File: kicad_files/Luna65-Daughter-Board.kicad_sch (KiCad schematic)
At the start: 39 parts, among them J1 TYPE-C-31-M12, J2 Molex Power, J3 JSTPH, Q1 TP0610T, U2 USBLC6-2SC6, U3 AP2112, U4 APX803L, U5 TPS61032RSAR, U6 LTC4095

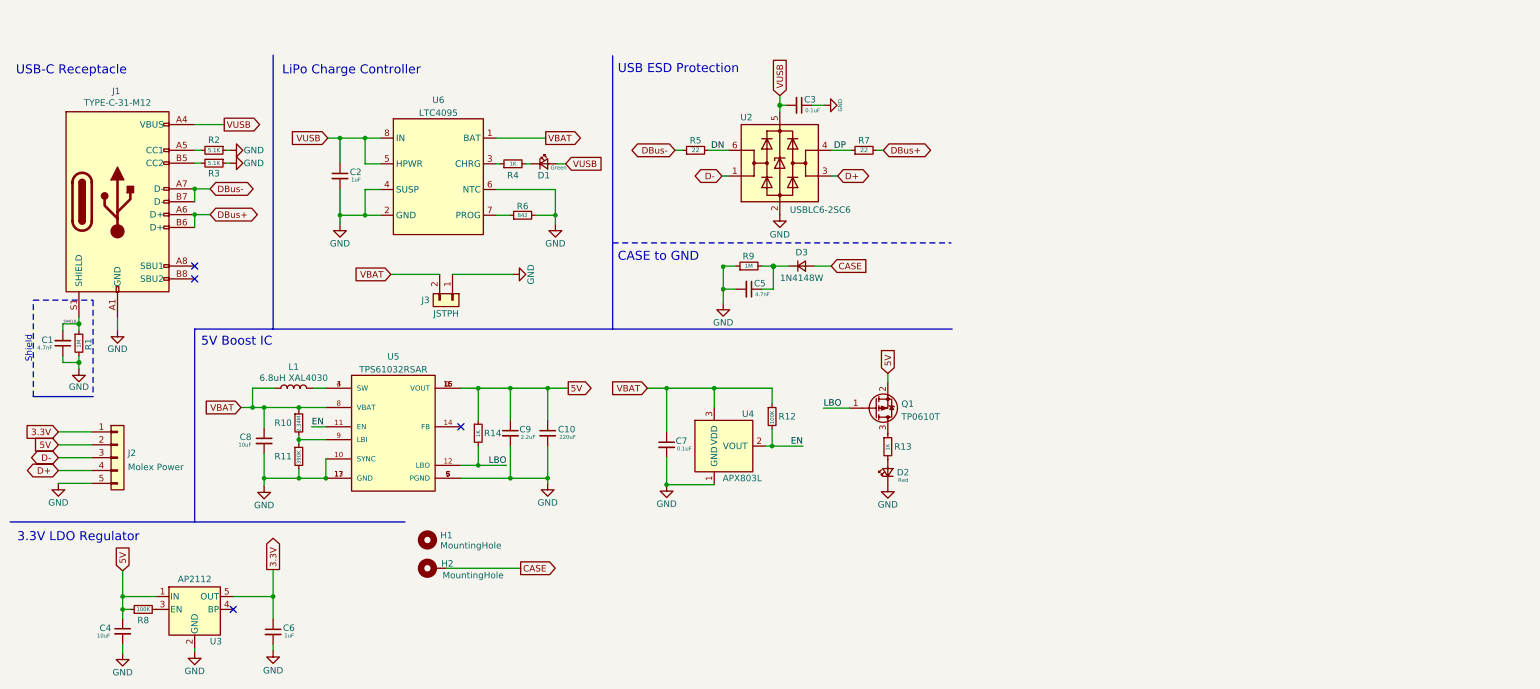
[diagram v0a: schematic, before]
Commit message: stuff
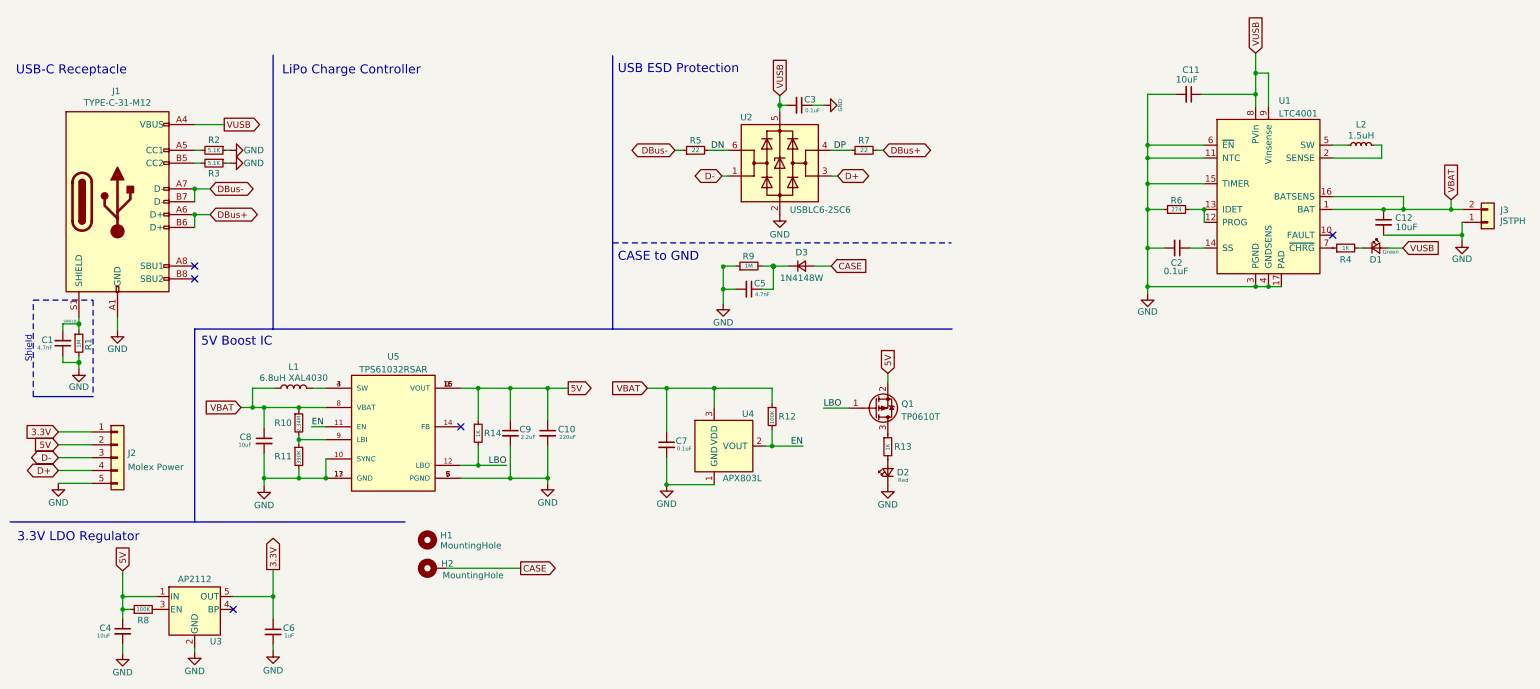
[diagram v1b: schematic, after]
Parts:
- removed U6: LTC4095, Package_DFN_QFN:DFN-8-1EP_2x2mm_P0.5mm_EP0.7x1.3mm, symbol LTC4095:LTC4095
- added C11, C12: 10uF, Capacitor_SMD:C_0603_1608Metric, symbol Device:C_Small
- added L2: 1.5uH, Inductor_SMD:L_0805_2012Metric, symbol Device:L_Small
- added U1: LTC4001, Package_DFN_QFN:QFN-16-1EP_4x4mm_P0.65mm_EP2.15x2.15mm, symbol Battery_Management:LTC4001
- C1, C3, C4, C5, C6, C7, C8, C9: footprint acheron_Components:C_0805_2012Metric -> Capacitor_SMD:C_0603_1608Metric
- C2: value 1uF -> 0.1uF; footprint acheron_Components:C_0805_2012Metric -> Capacitor_SMD:C_0603_1608Metric
- D1, D2: footprint LED_SMD:LED_1206_3216Metric_Pad1.42x1.75mm_HandSolder -> LED_SMD:LED_0805_2012Metric
- R1, R10, R11, R12, R13, R14, R2, R3, R4, R5, R7, R8, R9: footprint Resistor_SMD:R_0805_2012Metric -> Resistor_SMD:R_0603_1608Metric
- R6: value 842 -> 274; footprint Resistor_SMD:R_0805_2012Metric -> Resistor_SMD:R_0603_1608Metric
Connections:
- net GND: now also R6.1, C11.2, C12.2, U1.11 (NTC), U1.15 (TIMER), U1.17 (PAD), U1.3 (PGND), U1.4 (GNDSENS), U1.6 (~{EN}); no longer R6.2
- net VBAT: now also C12.1, U1.1 (BAT), U1.16 (BATSENS)
- net VUSB: now also C11.1, U1.8 (PVin), U1.9 (Vinsense); no longer C2.1
- net at R4.1: now also U1.7 (~{CHRG})
- new net: L2.1, U1.5 (SW)
- new net: L2.2, U1.2 (SENSE)
- new net: R6.2, U1.12 (PROG), U1.13 (IDET)
- new net: C2.1, U1.14 (SS)
- no-connect marks 4 -> 5
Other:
- moved on the sheet: D1, R4
